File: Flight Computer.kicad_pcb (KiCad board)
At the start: 4 copper layers, 39 x 80 mm, 132 parts, among them J1 Screw Switches, J10 Micro_SD_Card, J2 Pyro Channels, J3 Serial Wire Debug, J4 JST-PH, J7 USB_C_Receptacle_USB2.0, J8 External UART, J9 External I2C, Q1 MMBT2222A, Q2 AO3400A, Q3 AO3400A, Q4 AO3401A, Q5 AO3400A, Q6 AO3400A, Q7 AO3400A, Q8 AO3400A, Q9 AO3401A, U1 STM32L476VETx, U11 SAM-M8Q, U2 USBLC6-2SC6, U7 W25Q128JVSIQ, U8 TPS61230DRC, U9 LM3670MF, Y1 16MHz

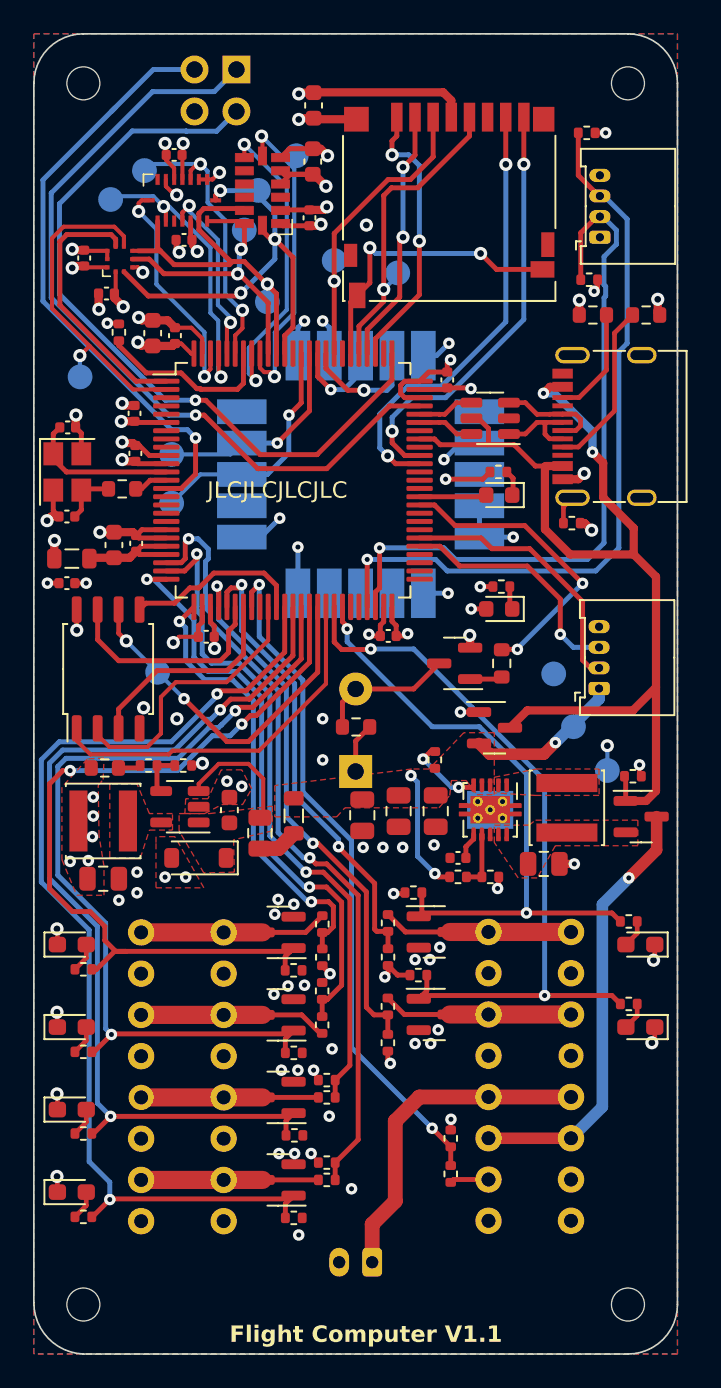
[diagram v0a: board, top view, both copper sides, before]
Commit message: Updated with notes from Erik Welsh
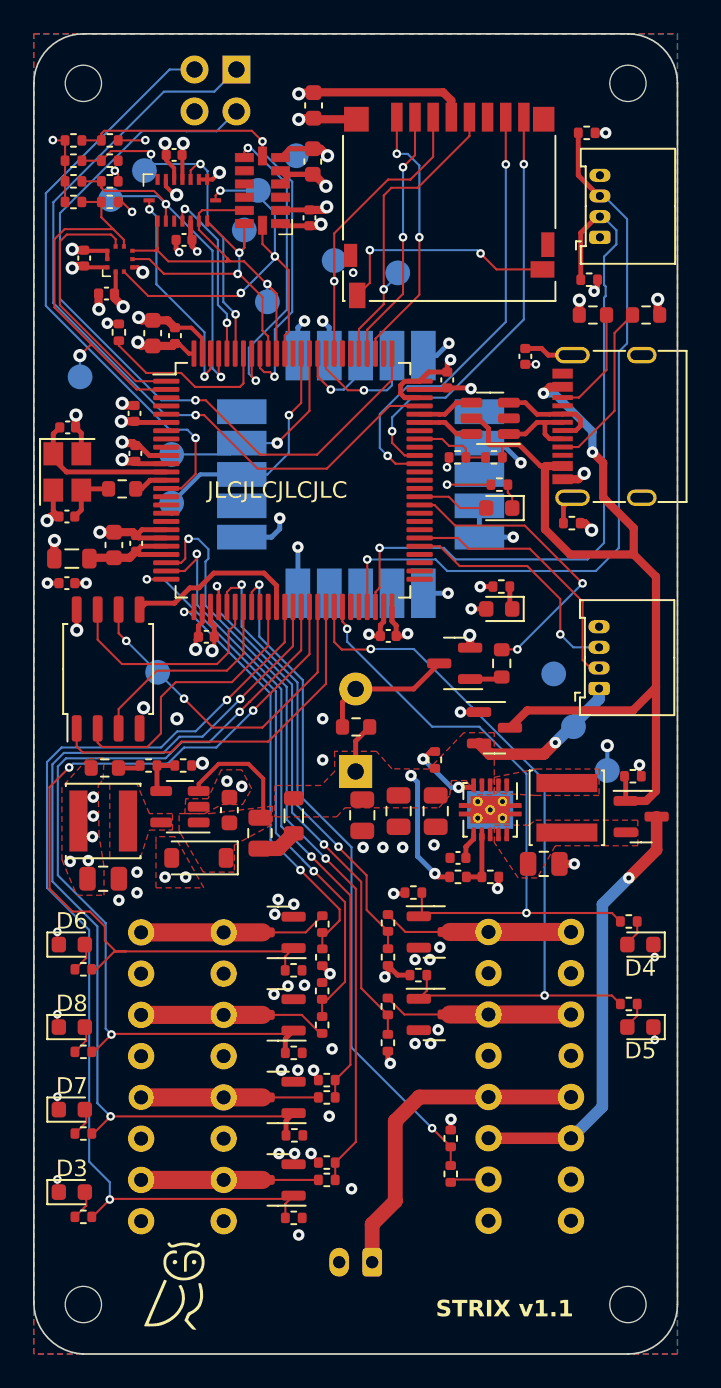
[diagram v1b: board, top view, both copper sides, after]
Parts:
- added C25: 0.01u, Capacitor_SMD:C_0402_1005Metric, F.Cu at (162.6, 83.1)
- added G***: LOGO, LOGO, F.Cu at (141.5, 139.3)
- added G***: LOGO, LOGO, B.Cu at (140.0, 109.0)
- added R45: 51k, Resistor_SMD:R_0402_1005Metric, F.Cu at (160.7, 89.2)
- added R46: 200k, Resistor_SMD:R_0402_1005Metric, F.Cu at (158.5, 89.2)
- added R48: 0, Resistor_SMD:R_0402_1005Metric, F.Cu at (135.2, 70.0)
- added R49: 0, Resistor_SMD:R_0402_1005Metric, F.Cu at (137.4, 70.0)
- added R50: 0, Resistor_SMD:R_0402_1005Metric, F.Cu at (135.2, 72.5)
- added R51: 0, Resistor_SMD:R_0402_1005Metric, F.Cu at (137.4, 72.5)
- added R52: 0, Resistor_SMD:R_0402_1005Metric, F.Cu at (135.2, 71.2)
- added R53: 0, Resistor_SMD:R_0402_1005Metric, F.Cu at (137.4, 71.2)
- added R54: 0, Resistor_SMD:R_0402_1005Metric, F.Cu at (135.2, 73.7)
- added R55: 0, Resistor_SMD:R_0402_1005Metric, F.Cu at (137.4, 73.7)
- D1: value Green -> Blue
- D2: value Red -> Green
- D3, D4, D5, D6, D7, D8: footprint LED_SMD:LED_0603_1608Metric_Pad1.05x0.95mm_HandSolder -> LED_SMD:LED_0603_1608Metric
- H1, H2, H3, H4: footprint MountingHole:MountingHole_2mm -> MountingHole:MountingHole_2.2mm_M2
- R17, R24, R36, R37, R38, R39, R40, R41: value 1.5k -> 1k
- moved D1 0.79 mm to (161.0, 92.2)
- moved R17 0.77 mm to (161.0, 90.8)
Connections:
- U1 pad 68: /USB 5V in -> Net-(U1-PA9)
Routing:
- net Net-(J7-SHIELD): track 1.77 -> 21.8 mm
- net /Chip Select High G Accel: track 19.1 -> 30.0 mm
- net /Chip Select Low G Accel: track 17.9 -> 23.9 mm
- net +3.3V: track 57.3 -> 62.4 mm, vias 29 -> 30
- net Net-(U1-PA9): track 0.00 -> 4.76 mm
- net /Chip Select Low G Gyro: track 17.6 -> 22.4 mm, vias 2 -> 3
- net /USB 5V in: track 64.6 -> 61.2 mm
- net /SD Card Detect: track 17.9 -> 14.6 mm
- net GND: track 91.9 -> 94.9 mm, vias 86 -> 91
- net /Chip Select Altimeter: track 20.8 -> 23.5 mm
- net /Pyro B Continuity Voltage: track 41.2 -> 39.6 mm
- net /Pyro D Continuity Voltage: track 27.1 -> 25.9 mm
- net /Pyro C Continuity Voltage: track 35.2 -> 34.0 mm
- net /NRST: track 36.7 -> 35.7 mm
- net /Pyro Channel A Trigger: track 63.0 -> 62.0 mm
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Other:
- board text added: "2023/10/13"
- board text added: "STRIX v1.1"
- board text removed: "2023/10/4"
- board text removed: "Flight Computer V1.1"

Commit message: KiCAD is broken
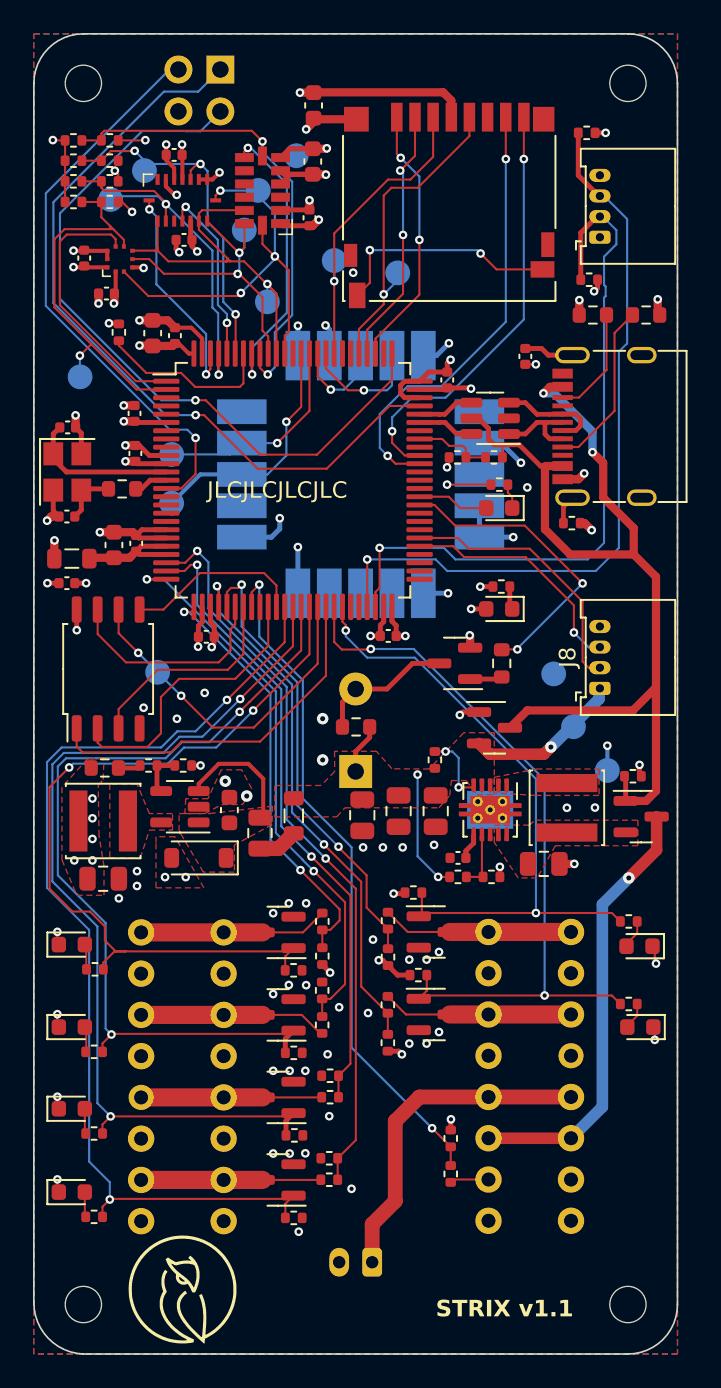
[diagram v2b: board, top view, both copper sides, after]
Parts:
- removed the G*** at (141.5, 139.3)
- removed the G*** at (140.0, 109.0)
- added G***: LOGO, LOGO, F.Cu at (141.8, 139.6)
- added G***: LOGO, LOGO, B.Cu at (141.1, 109.8)
- moved J3 0.97 mm to (144.1, 65.7)
- moved R39 0.70 mm to (136.5, 120.2)
- moved R36 0.65 mm to (136.4, 135.2)
- moved R40 0.65 mm to (136.4, 130.2)
- moved R41 0.65 mm to (136.4, 125.2)
- moved R8 0.33 mm to (150.8, 126.7)
- moved R6 0.30 mm to (150.7, 131.7)
- moved R7 0.20 mm to (150.8, 128.0)
- moved R15 0.16 mm to (150.3, 117.3)
- moved R4 0.15 mm to (150.7, 132.9)
- moved R11 0.14 mm to (154.3, 117.2)
- moved D4 0.11 mm to (169.5, 118.8)
- moved R13 0.10 mm to (154.2, 122.3)
- moved R16 0.07 mm to (150.3, 119.4)
- moved R22 0.07 mm to (160.5, 114.6)
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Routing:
- net GND: track 94.9 -> 92.2 mm, vias 91 -> 98
- net +3.3V: track 62.4 -> 60.1 mm
- net /Pyro A Continuity Voltage: track 46.6 -> 44.7 mm
- net /Pyro B Continuity Voltage: track 39.6 -> 38.4 mm
- net /High G Interrupt: track 18.7 -> 17.6 mm
- net /SWDIO: track 48.5 -> 47.5 mm
- net /SWCLK: track 45.9 -> 45.0 mm
- net /NRST: track 35.7 -> 34.7 mm
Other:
- board text added: "GND"
- board text added: "GND SCL SDA +3.3"
- board text added: "GND TX RX +5"
- board text added: "gnd"
- board text added: "nrst"
- board text added: "swclk"
- board text added: "swdio"
- board text removed: "13"
- board text removed: "14"
- board text removed: "6"
- board text removed: "7"
- board text removed: "8"
- board text removed: "9"
- board text removed: "Gnd SCL SDA +3.3"
- board text removed: "Gnd TX RX +5"
- board text removed: "MISO"
- board text removed: "MOSI"
- board text removed: "NRST"
- board text removed: "QSPI Clk"
- board text removed: "SCK"
- board text removed: "SWCLK"
- board text removed: "SWDIO"
